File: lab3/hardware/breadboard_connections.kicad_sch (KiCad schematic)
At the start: 40 parts, among them Q1 2N3906, Q2 2N3906, SW1 SW_SPST, SW2 SW_SPST, SW3 SW_SPST, SW4 SW_SPST

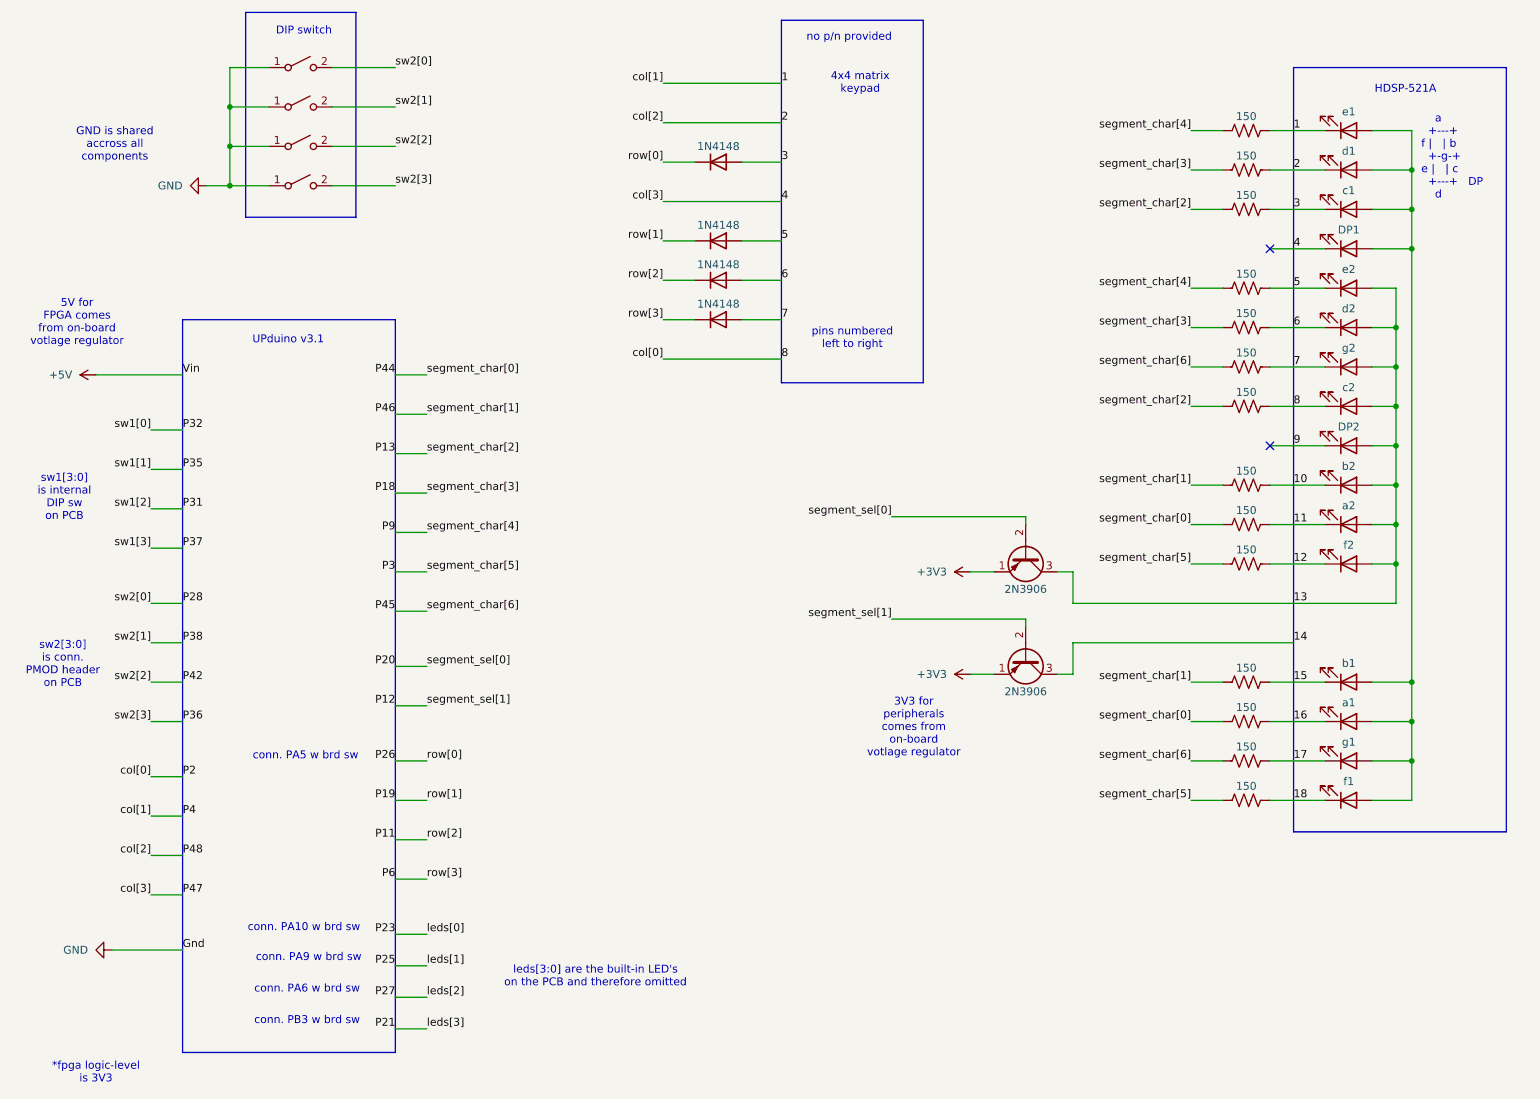
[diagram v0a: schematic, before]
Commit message: Lab 3 circuit diagram
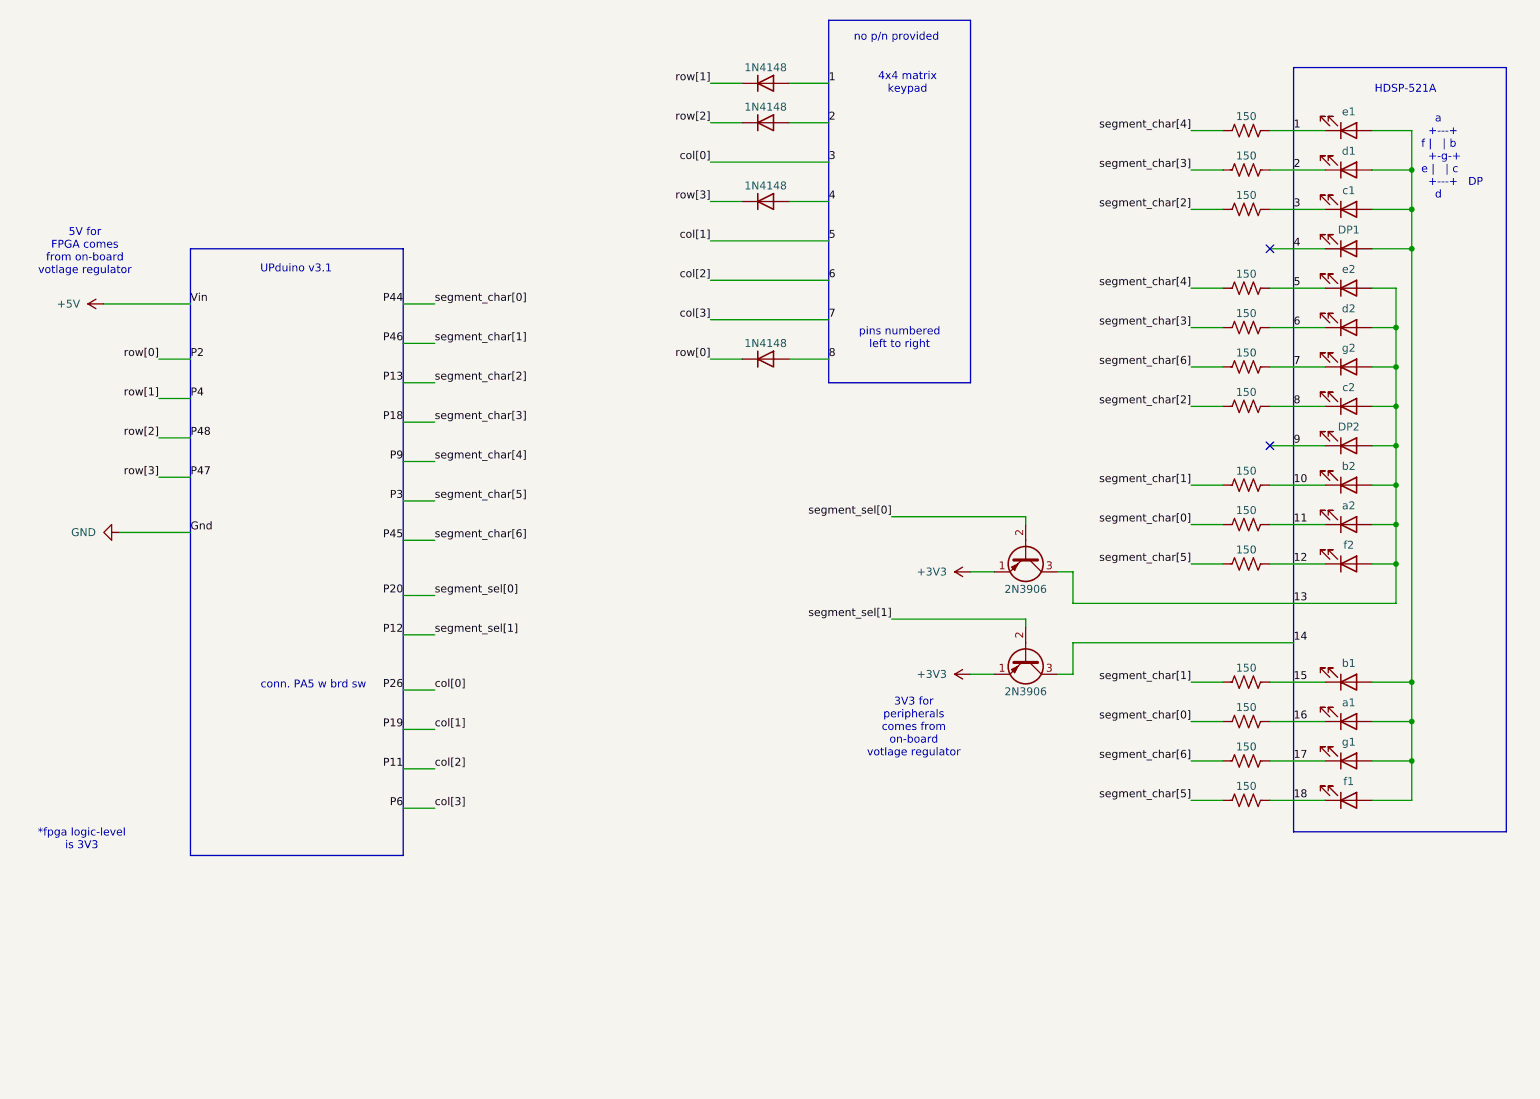
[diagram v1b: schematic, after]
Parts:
- removed SW1, SW2, SW3, SW4: SW_SPST, symbol Switch:SW_SPST
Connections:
- net 1: now also D13.2 (A)
- net 2: now also D14.2 (A)
- net 3: no longer D13.2 (A)
- net 4: now also D19.2 (A)
- net 5: no longer D14.2 (A)
- net 6: no longer D19.2 (A)
- net 7: no longer D20.2 (A)
- net 8: now also D20.2 (A)
- net P11 renamed P47
- net P19 renamed P48
- net P26 renamed P4
- net P6 renamed P2
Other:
- note removed: "DIP switch"
- note removed: "GND is shared accross all components"
- note removed: "conn. PA10 w brd sw"
- note removed: "conn. PA6 w brd sw"
- note removed: "conn. PA9 w brd sw"
- note removed: "conn. PB3 w brd sw"
- note removed: "leds[3:0] are the built-in LED's on the PCB and therefore omitted"
- note removed: "sw1[3:0] is internal DIP sw on PCB"
- note removed: "sw2[3:0] is conn. PMOD header on PCB"
